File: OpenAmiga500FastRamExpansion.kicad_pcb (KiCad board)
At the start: 2 copper layers, 99.7 x 71.2 mm, 35 parts, among them J1 68000_SOCKET, P1 JTAG_CONNECTOR, P99 OSHW_LOGO, U1 68000D, U2 74LS157, U3 74LS157, U4 ATF1502AS-10JU44, U5 HYB5118160BSJ, U6 HYB5118160BSJ, U7 HYB5118160BSJ, U8 HYB5118160BSJ

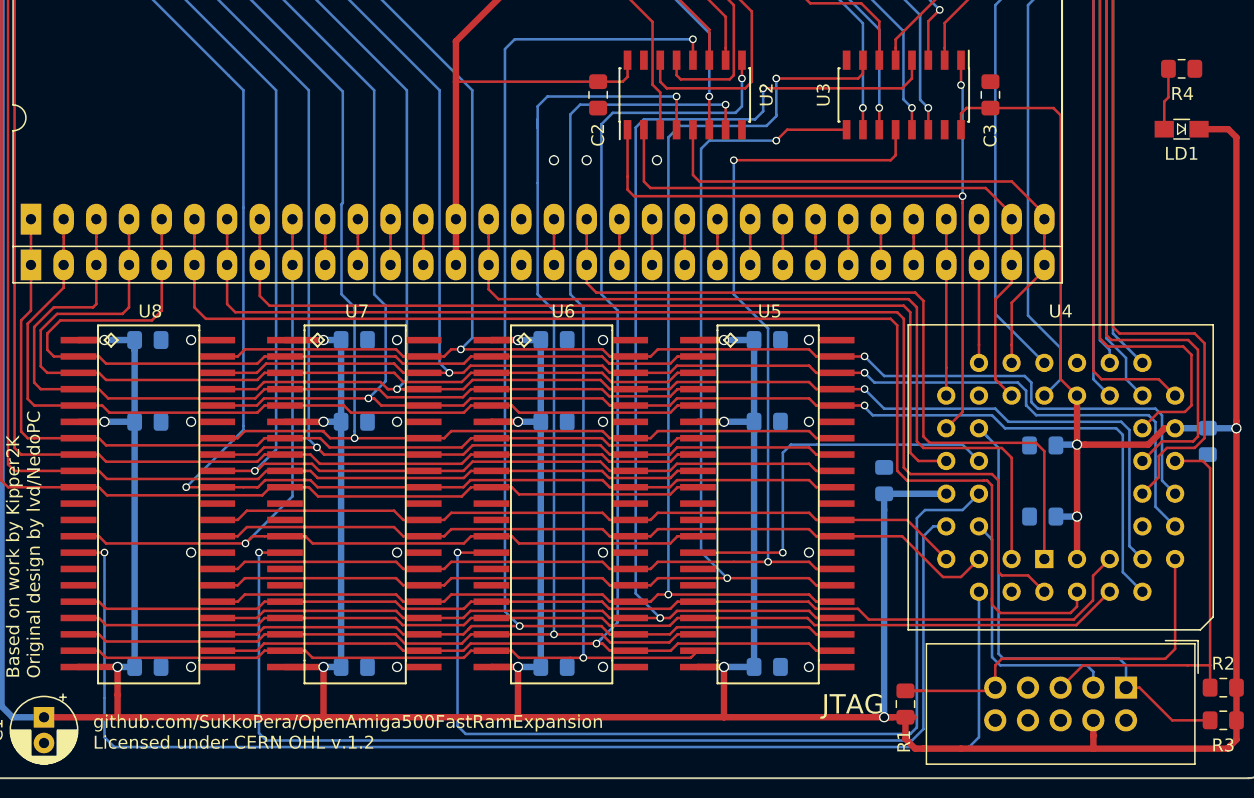
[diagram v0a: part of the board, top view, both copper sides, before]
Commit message: Refinements here and there
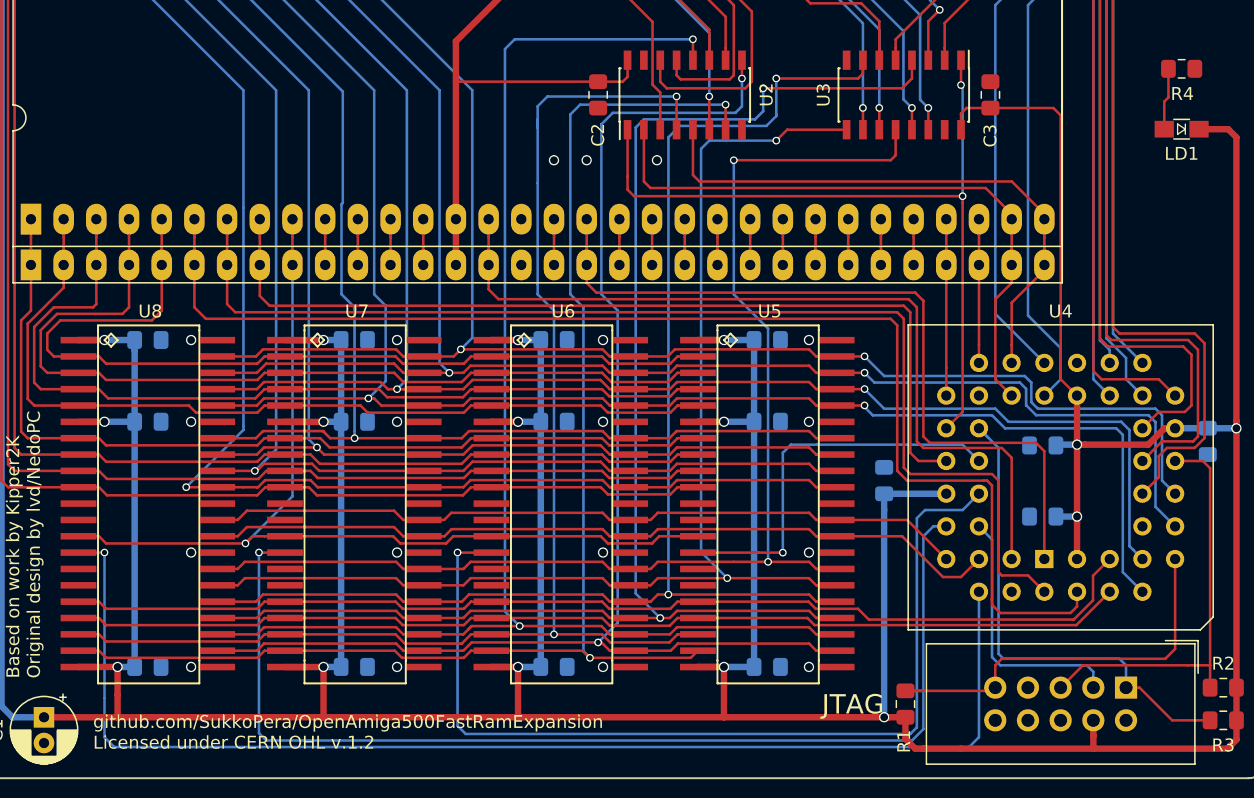
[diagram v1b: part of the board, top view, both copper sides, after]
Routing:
- net /ma4: track 106.7 -> 106.1 mm
